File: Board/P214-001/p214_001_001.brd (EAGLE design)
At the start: 70.8 x 71.1 mm, 24 parts, among them IC1 74LS07N

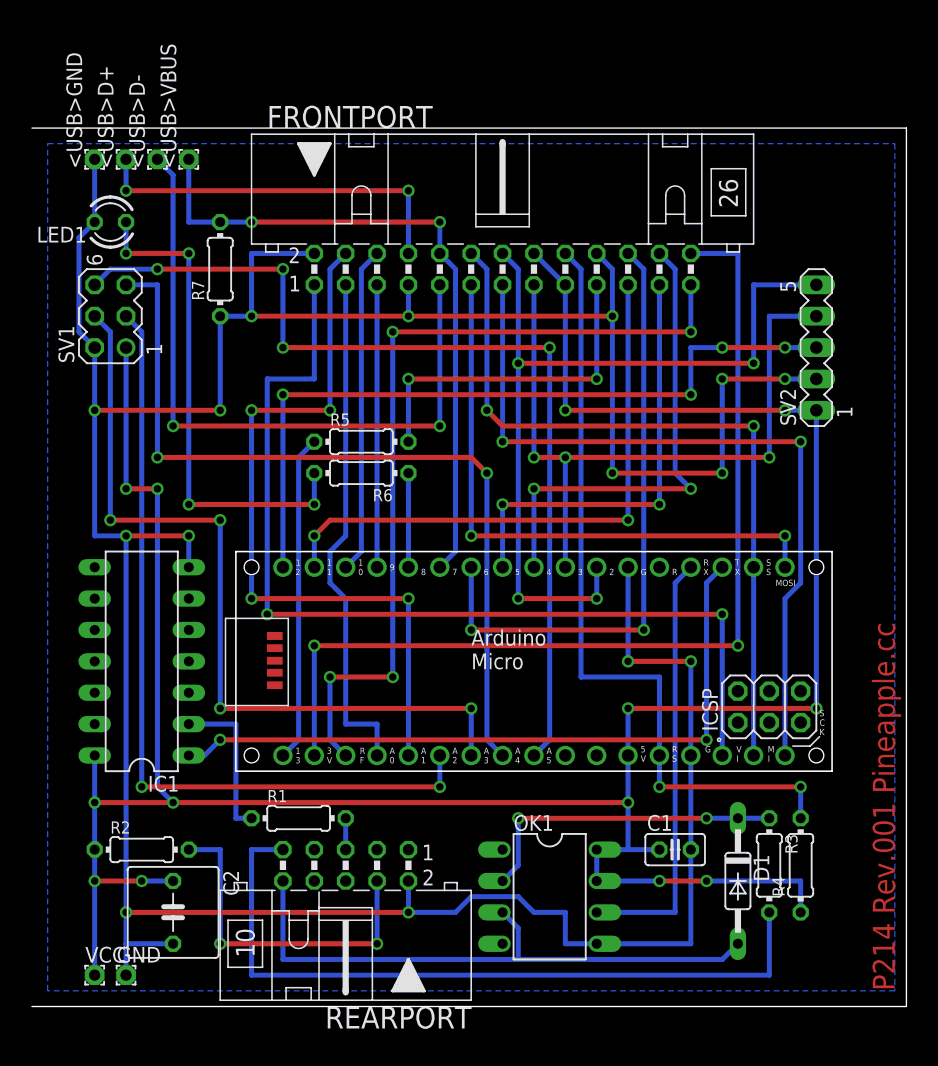
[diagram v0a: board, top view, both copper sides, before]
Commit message: new design.
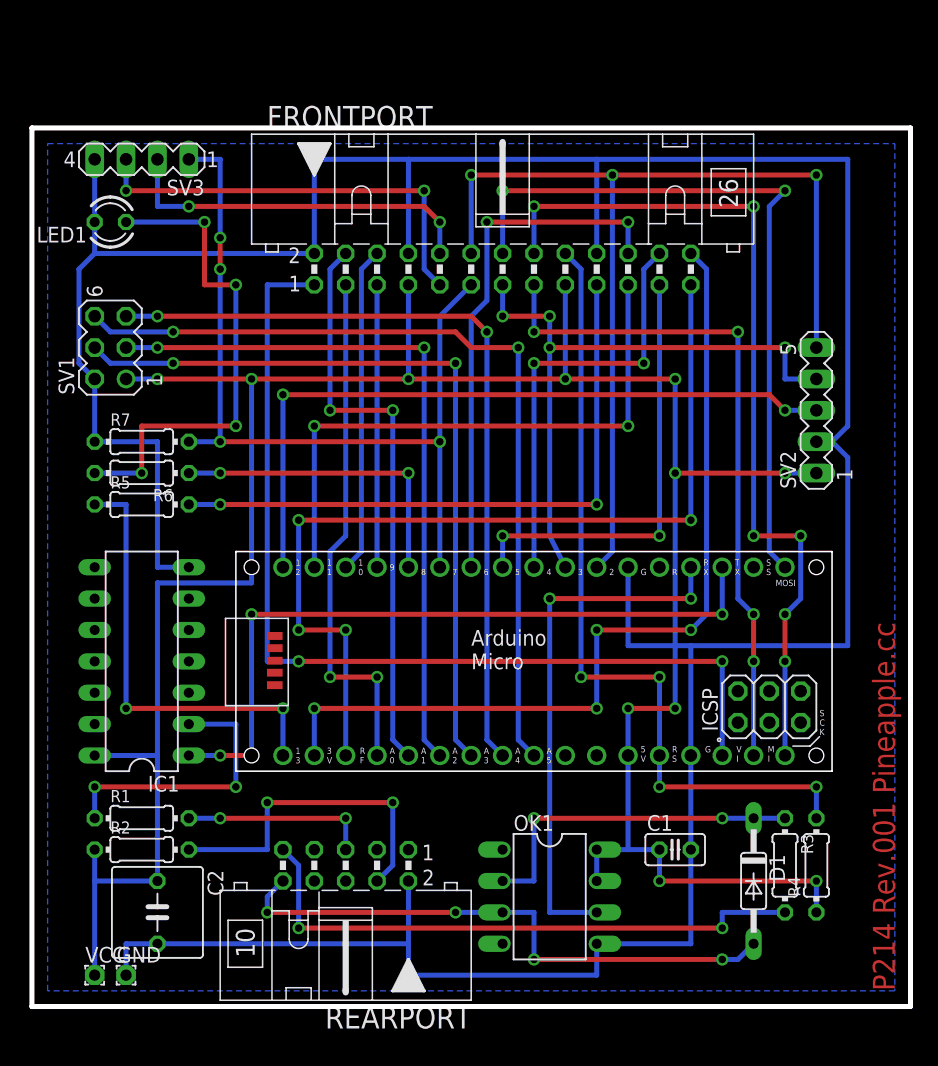
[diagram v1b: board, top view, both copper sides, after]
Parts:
- removed <USB>D+, <USB>D-, <USB>GND, <USB>VBUS: (no value), wirepad:1,6/0,9
- added SV3: USB, con-lstb:MA04-1
- R7: value (none) -> 10k
- SV1: value (none) -> Analog
- SV2: value (none) -> RTC
- moved R5 18.5 mm to (8.89, 40.6)
- moved R6 17.8 mm to (8.89, 43.2)
- moved R7 15.3 mm to (8.89, 45.7), turned to 0 degrees
- moved R1 12.7 mm to (8.89, 15.2)
- moved SV2 5.08 mm to (63.5, 48.3)
- moved SV1 2.54 mm to (6.35, 53.3)
- moved D1 1.27 mm to (58.4, 10.2)
- moved R3 1.27 mm to (61.0, 11.4)
- moved R4 1.27 mm to (63.5, 11.4)
- moved C2 1.27 mm to (10.2, 7.62)
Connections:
- removed net N$25: <USB>VBUS.1, FRONTPORT.10, PCB1.D7, R7.2
- new net N$39: FRONTPORT.10, SV3.2
- net GND: now also FRONTPORT.8, SV3.4; no longer <USB>GND.1, FRONTPORT.7
- net N$14: now also FRONTPORT.14; no longer FRONTPORT.11
- net N$15: now also FRONTPORT.15; no longer FRONTPORT.12
- net N$16: now also FRONTPORT.16; no longer FRONTPORT.13
- net N$17: now also FRONTPORT.12; no longer FRONTPORT.14
- net N$18: now also FRONTPORT.13; no longer FRONTPORT.15
- net N$22: now also SV3.3; no longer <USB>D-.1
- net N$24: now also FRONTPORT.11, PCB1.D7, R7.2, SV3.1; no longer <USB>D+.1, FRONTPORT.8
- net VCC: now also FRONTPORT.7; no longer FRONTPORT.16
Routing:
- net N$25: track 54.4 -> 0.00 mm, vias 2 -> 0
- net N$24: track 30.5 -> 69.6 mm, vias 2 -> 4
- net N$39: track 0.00 -> 29.7 mm, vias 0 -> 2
- net N$19: track 27.9 -> 50.8 mm
- net N$22: track 55.1 -> 34.8 mm
- net N$35: track 7.62 -> 25.4 mm, vias 0 -> 2
- net N$11: track 60.2 -> 46.8 mm, vias 4 -> 2
- net N$17: track 67.8 -> 80.5 mm, vias 4 -> 3
- net N$5: track 2.54 -> 15.2 mm, vias 0 -> 2
- net N$6: track 59.7 -> 47.5 mm, vias 0 -> 2
- net VCC: track 218.7 -> 207.0 mm, vias 13 -> 11
- net N$14: track 48.3 -> 59.5 mm
- net N$2: track 12.7 -> 22.9 mm, vias 0 -> 2
- net N$20: track 26.5 -> 35.6 mm, vias 0 -> 2
- net N$8: track 34.8 -> 43.2 mm, vias 0 -> 2
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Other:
- board size 70.8 x 71.1 mm -> 71.1 x 71.1 mm
